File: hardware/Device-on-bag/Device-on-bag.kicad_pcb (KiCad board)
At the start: 2 copper layers, 51.4 x 37.2 mm, 4 parts, among them J1 Conn_01x12, J2 Conn_01x12

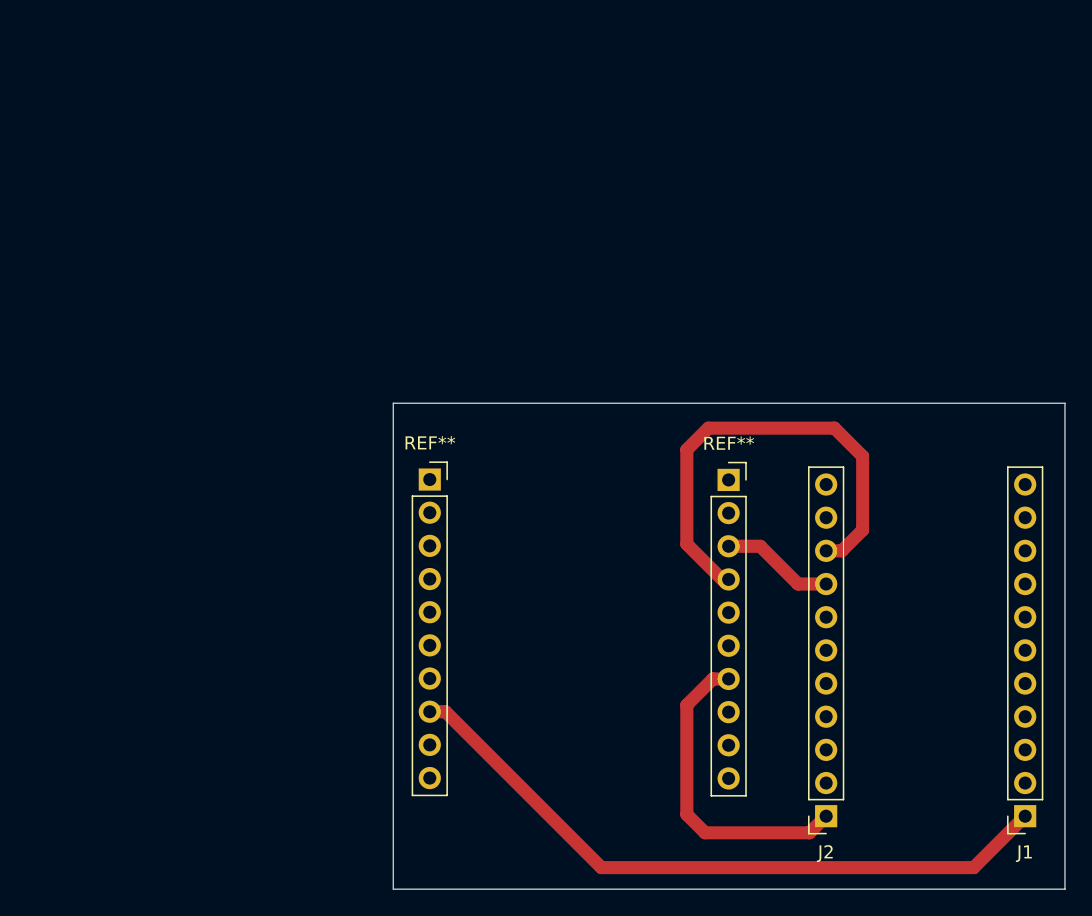
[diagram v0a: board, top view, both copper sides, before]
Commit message: update
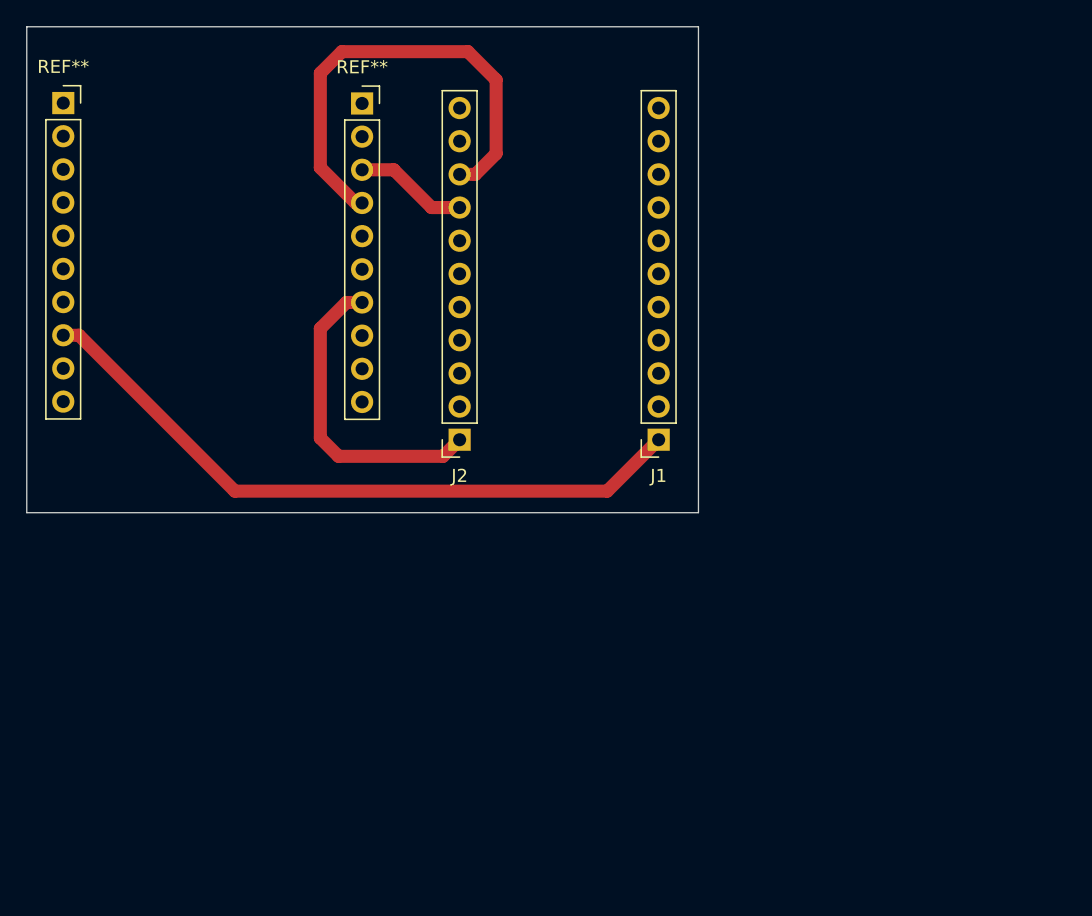
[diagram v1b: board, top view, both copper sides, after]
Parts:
- removed the REF** at (142.3, 84.1)
- removed the REF** at (119.4, 84.1)
- added REF**: PinSocket_1x10_P2.54mm_Vertical, Connector_PinSocket_2.54mm:PinSocket_1x10_P2.54mm_Vertical, F.Cu at (91.3, 55.2)
- added REF**: PinSocket_1x10_P2.54mm_Vertical, Connector_PinSocket_2.54mm:PinSocket_1x10_P2.54mm_Vertical, F.Cu at (114.2, 55.3)
- moved J1 40.2 mm to (136.9, 81.0)
- moved J2 40.2 mm to (121.7, 81.0)
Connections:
- J1 pad 1: 3v3 -> (no net)
- J1 pad 10: unconnected-(J1-Pad10) -> (no net)
- J1 pad 11: unconnected-(J1-Pad11) -> (no net)
- J1 pad 2: unconnected-(J1-Pad2) -> (no net)
- J1 pad 3: unconnected-(J1-Pad3) -> (no net)
- J1 pad 4: unconnected-(J1-Pad4) -> (no net)
- J1 pad 5: unconnected-(J1-Pad5) -> (no net)
- J1 pad 6: unconnected-(J1-Pad6) -> (no net)
- J1 pad 7: unconnected-(J1-Pad7) -> (no net)
- J1 pad 8: unconnected-(J1-Pad8) -> (no net)
- J1 pad 9: unconnected-(J1-Pad9) -> (no net)
- J2 pad 1: GND -> (no net)
- J2 pad 10: unconnected-(J2-Pad10) -> (no net)
- J2 pad 11: unconnected-(J2-Pad11) -> (no net)
- J2 pad 2: unconnected-(J2-Pad2) -> (no net)
- J2 pad 3: unconnected-(J2-Pad3) -> (no net)
- J2 pad 4: unconnected-(J2-Pad4) -> (no net)
- J2 pad 5: unconnected-(J2-Pad5) -> (no net)
- J2 pad 6: unconnected-(J2-Pad6) -> (no net)
- J2 pad 7: unconnected-(J2-Pad7) -> (no net)
- J2 pad 8: SCL -> (no net)
- J2 pad 9: SDA -> (no net)
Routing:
- net (no net): track 0.00 -> 121.2 mm
- net 3v3: track 52.2 -> 0.00 mm
- net SDA: track 35.7 -> 0.00 mm
- net GND: track 24.7 -> 0.00 mm
- net SCL: track 8.67 -> 0.00 mm

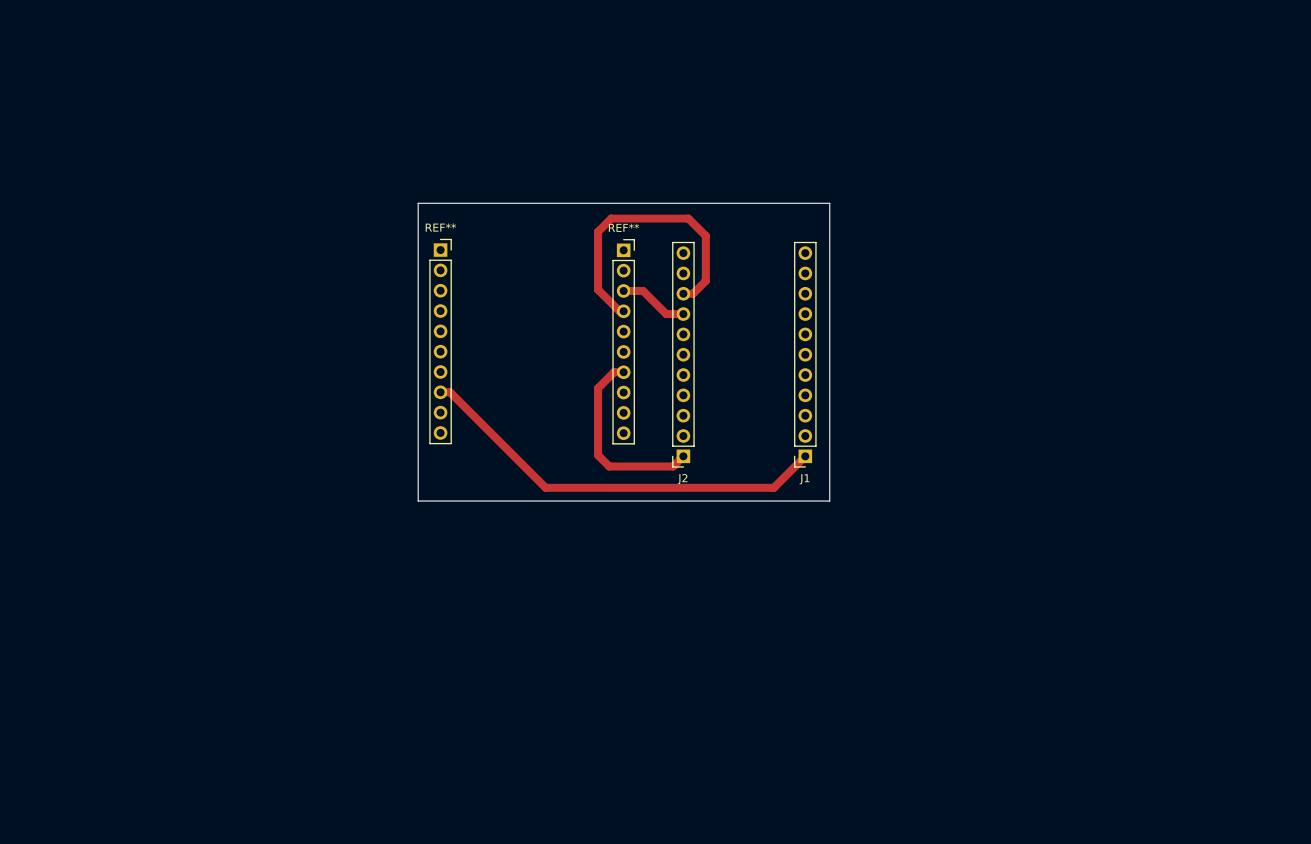
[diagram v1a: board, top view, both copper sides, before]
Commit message: update
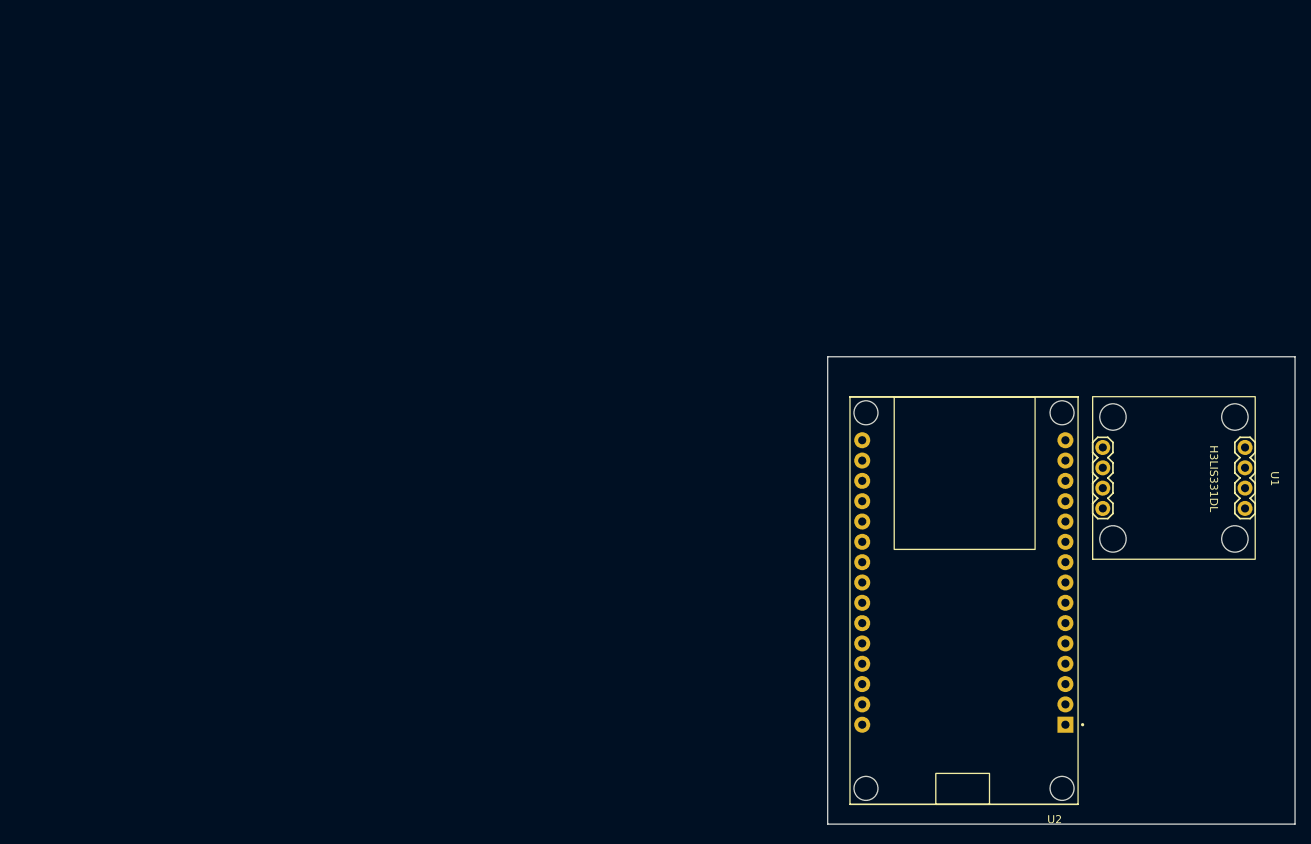
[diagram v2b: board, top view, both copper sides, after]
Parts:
- removed J1, J2: Conn_01x12, Connector_PinSocket_2.54mm:PinSocket_1x11_P2.54mm_Vertical
- removed REF** (x2): PinSocket_1x10_P2.54mm_Vertical, Connector_PinSocket_2.54mm:PinSocket_1x10_P2.54mm_Vertical
- added U1: SparkFun_SEN-14480_H3LIS331DL, SparkFun_Tri_Axis_Accel_Breakout-H3LIS331DL:SparkFun_Tri_Axis_Accel_Breakout-H3LIS331DL, F.Cu at (182.9, 83.8)
- added U2: ESP32-DEVKIT-V1, ESP32-DEVKIT-V1:MODULE_ESP32_DEVKIT_V1, F.Cu at (156.7, 99.1)
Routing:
- net (no net): track 121.2 -> 0.00 mm
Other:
- board size 51.4 x 37.2 mm -> 58.4 x 58.4 mm

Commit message: update
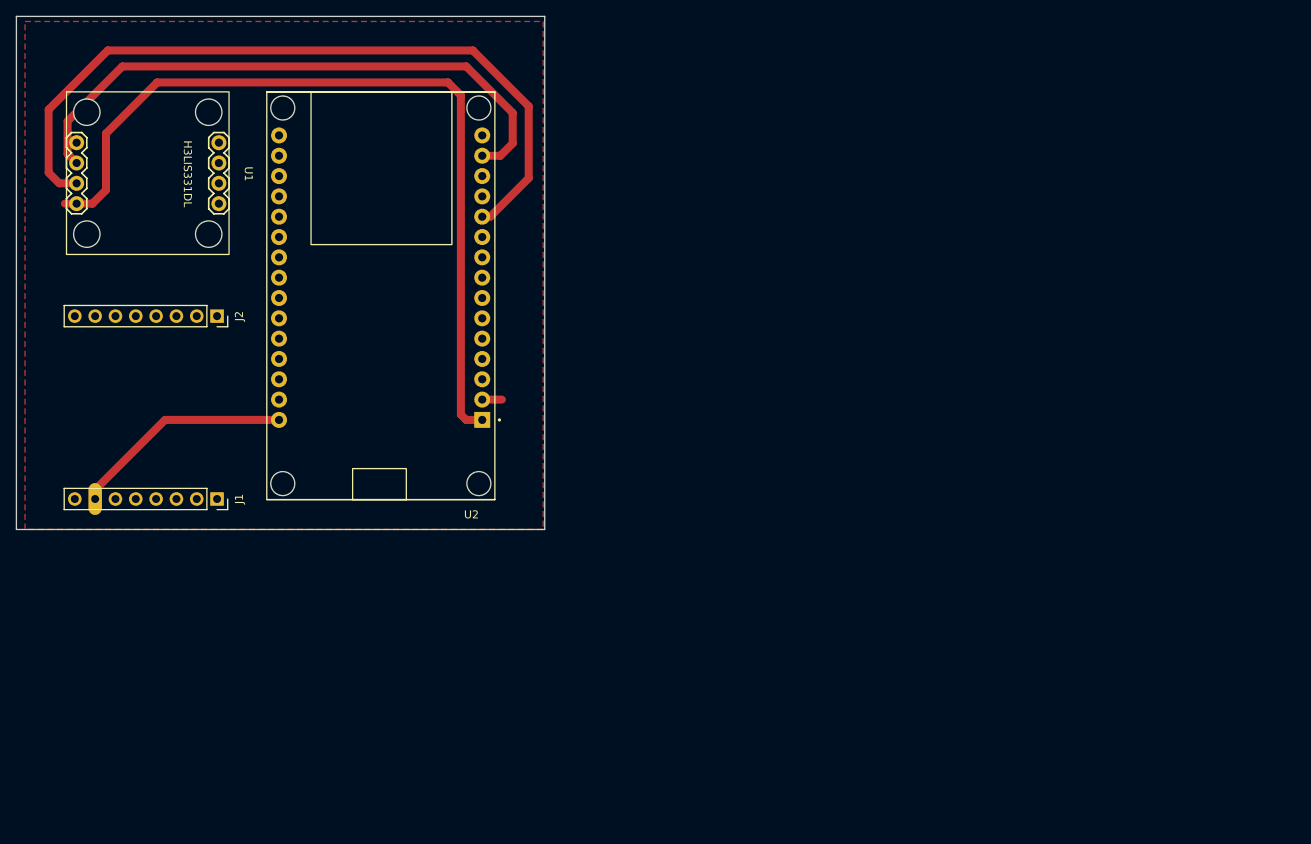
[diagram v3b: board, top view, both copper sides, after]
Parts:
- added J1: Conn_01x08, Connector_PinSocket_2.54mm:PinSocket_1x08_P2.54mm_Vertical, F.Cu at (63.4, 86.4)
- added J2: Conn_01x08, Connector_PinSocket_2.54mm:PinSocket_1x08_P2.54mm_Vertical, F.Cu at (63.4, 63.5)
- moved U1 133.8 mm to (54.6, 45.7)
- moved U2 82.3 mm to (83.8, 61.0)
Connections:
- U2 pad 11: unconnected-(U2-Pad11) -> SDA
- U2 pad 14: unconnected-(U2-Pad14) -> SCL
- U2 pad 2: unconnected-(U2-Pad2) -> GND
- U2 pad 21: SDA -> unconnected-(U2-Pad21)
- U2 pad 22: SCL -> unconnected-(U2-Pad22)
- U2 pad 29: GND -> unconnected-(U2-Pad29)
- U2 pad 30: unconnected-(U2-Pad30) -> Vin
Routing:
- net 3.3V: track 0.00 -> 103.4 mm
- net SDA: track 0.00 -> 94.7 mm
- net SCL: track 0.00 -> 74.8 mm
- net Vin: track 0.00 -> 29.0 mm
- net GND: track 0.00 -> 2.46 mm
- added copper zone on F.Cu, net GND
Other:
- board size 58.4 x 58.4 mm -> 66 x 64.1 mm
